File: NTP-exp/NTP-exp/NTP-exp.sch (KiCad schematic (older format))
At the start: 19 parts

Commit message: exp pcb
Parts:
- removed Q? (x2): 2N3904, Package_TO_SOT_SMD:SOT-23, symbol Transistor_BJT:2N3904
- removed R?: 10k, Resistor_SMD:R_0805_2012Metric_Pad1.15x1.40mm_HandSolder, symbol Device:R_US
- removed R? (x2): 1k, Resistor_SMD:R_0805_2012Metric_Pad1.15x1.40mm_HandSolder, symbol Device:R_US
- removed R?: 200, Resistor_SMD:R_0805_2012Metric_Pad1.15x1.40mm_HandSolder, symbol Device:R_US
- added D3, D4, D5, D6, D7: LED, LED_THT:LED_D3.0mm_FlatTop, symbol Device:LED
- added J10, J11, J12, J13, J14, J15, J16, J17, J18, J4, J5, J6, J7, J8, J9: PJ301M-12, eurorack:PJ301M-12, symbol Eurorack:PJ301M-12
- added R1, R10, R15, R18, R19, R20, R23, R24, R25, R28, R29, R30, R33, R34, R4, R5, R6, R9: 51, Resistor_SMD:R_0805_2012Metric_Pad1.15x1.40mm_HandSolder, symbol Device:R_US
- added R16, R21, R26, R31, R7: 10m, Resistor_SMD:R_0805_2012Metric_Pad1.15x1.40mm_HandSolder, symbol Device:R_US
- added R17, R22, R27, R3, R32, R8: 1k, Resistor_SMD:R_0805_2012Metric_Pad1.15x1.40mm_HandSolder, symbol Device:R_US
- added SW2: SW_Rotary3x4, Potentiometer_THT:Potentiometer_Alpha_RD901F-40-00D_Single_Vertical, symbol Switch:SW_Rotary3x4
- added U1, U2, U4, U5, U6, U7: TL074, Package_DIP:DIP-14_W7.62mm_Socket, symbol Amplifier_Operational:TL074
- D2: renamed from D?; footprint Display_7Segment:7SegmentLED_LTS6760_LTS6780 -> Display_7Segment:AFF_2x7SEG-DIGIT_10mm
- R2: renamed from R?; value 1k -> 10m
- SW1: renamed from SW?; footprint (none) -> Potentiometer_THT:Potentiometer_Alpha_RD901F-40-00D_Single_Vertical
- U3: renamed from U?; footprint Package_DIP:DIP-28_W7.62mm -> Package_DIP:DIP-28_W7.62mm_Socket
- gave numbers to parts that had none: 9
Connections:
- net labels added: STr4, STr5, STr6
- wire segments 25 -> 176
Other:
- moved on the sheet: D1, D2, H1, J1, J2, J3, R11, R12, R13, R14, R2, SW1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

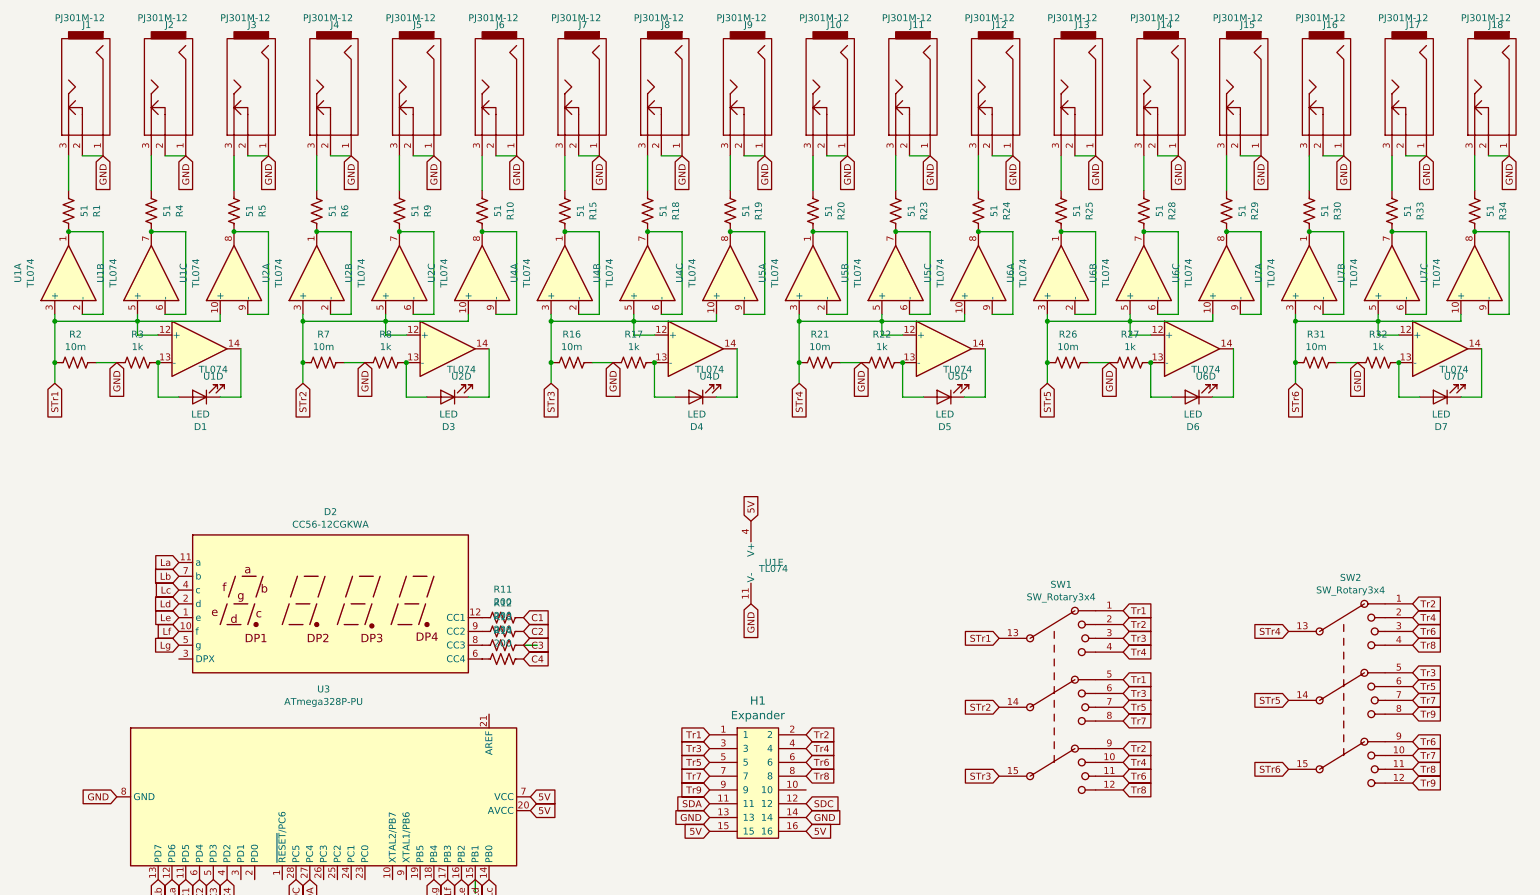
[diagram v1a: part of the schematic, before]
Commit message: designing
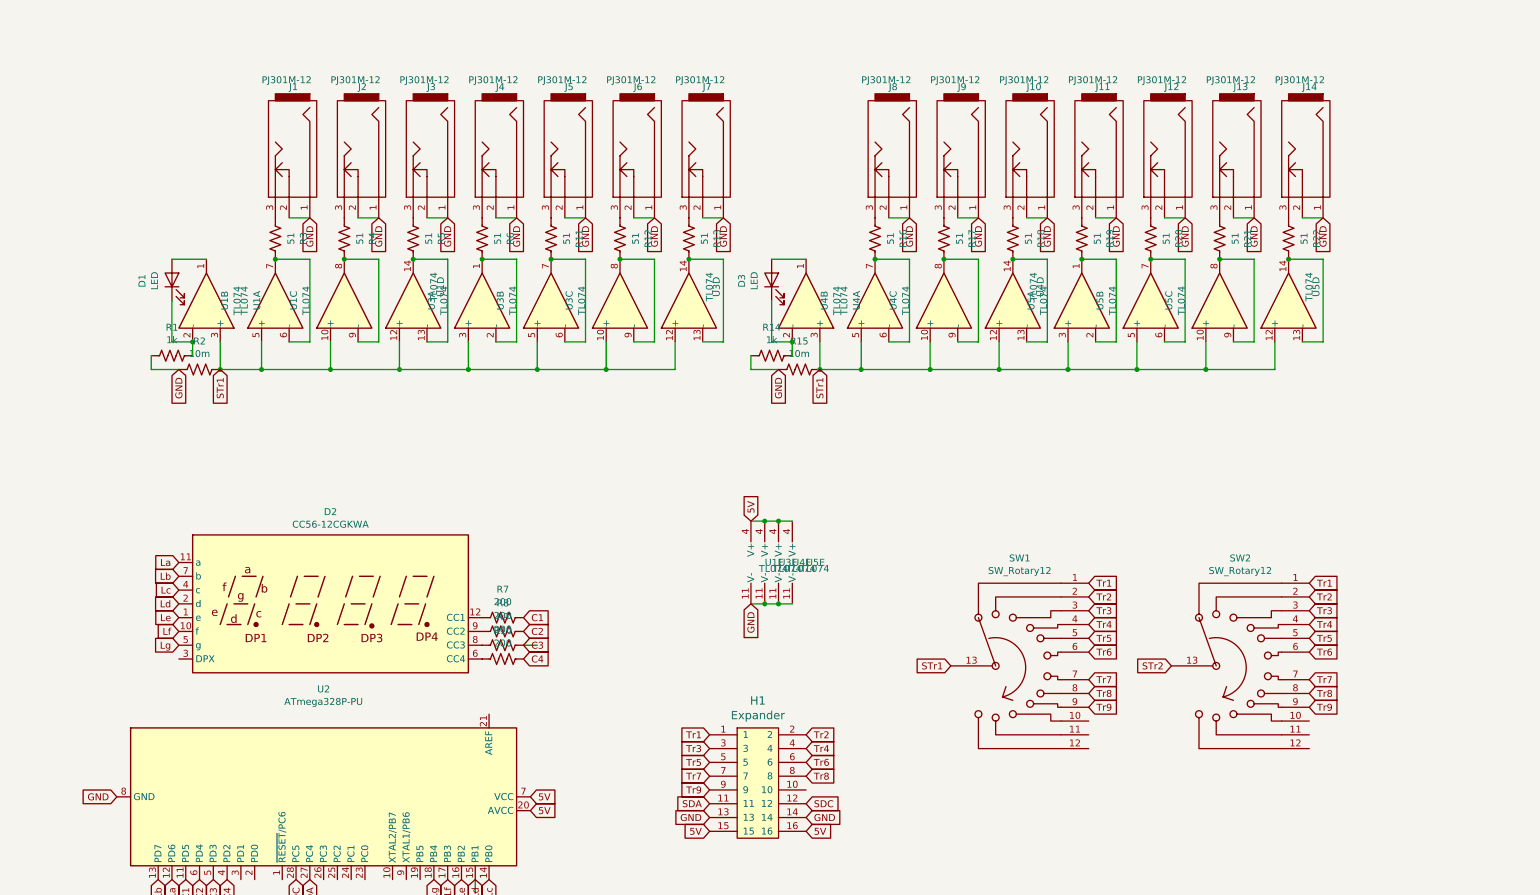
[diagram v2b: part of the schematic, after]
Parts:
- removed D4, D5, D6, D7: LED, LED_THT:LED_D3.0mm_FlatTop, symbol Device:LED
- removed J15, J16, J17, J18: PJ301M-12, eurorack:PJ301M-12, symbol Eurorack:PJ301M-12
- removed R10, R23, R24, R25, R28, R29, R30, R33, R34, R9: 51, Resistor_SMD:R_0805_2012Metric_Pad1.15x1.40mm_HandSolder, symbol Device:R_US
- removed R26, R31, R7: 10m, Resistor_SMD:R_0805_2012Metric_Pad1.15x1.40mm_HandSolder, symbol Device:R_US
- removed R27, R32, R8: 1k, Resistor_SMD:R_0805_2012Metric_Pad1.15x1.40mm_HandSolder, symbol Device:R_US
- removed SW1, SW2: SW_Rotary3x4, Potentiometer_THT:Potentiometer_Alpha_RD901F-40-00D_Single_Vertical, symbol Switch:SW_Rotary3x4
- removed U2, U6, U7: TL074, Package_DIP:DIP-14_W7.62mm_Socket, symbol Amplifier_Operational:TL074
- added R11, R12, R13: 51, Resistor_SMD:R_0805_2012Metric_Pad1.15x1.40mm_HandSolder, symbol Device:R_US
- added R14: 1k, Resistor_SMD:R_0805_2012Metric_Pad1.15x1.40mm_HandSolder, symbol Device:R_US
- added SW1, SW2: SW_Rotary12, symbol Switch:SW_Rotary12
- added U3: TL074, Package_DIP:DIP-14_W7.62mm_Socket, symbol Amplifier_Operational:TL074
- added unit 5 of U4
- added unit 5 of U5
- R1: value 51 -> 1k
- R15: value 51 -> 10m
- R16, R21: value 10m -> 51
- R17, R22, R3: value 1k -> 51
- renumbered R14 to R10, R11 to R7, R12 to R8, R13 to R9, U3 to U2
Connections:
- net 5V: now also U3.4 (V+), U4.4 (V+), U5.4 (V+)
- net GND: now also R1.2, R15.2, R2.2, R14.2, U3.11 (V-), U4.11 (V-), U5.11 (V-); no longer R16.1, R17.2, R2.1, R21.1, R22.2, R3.2
- net STr1: now also R15.1, R2.1, U4.10 (+), U4.12 (+), U4.3 (+), U4.5 (+), U5.10 (+), U5.12 (+), U5.3 (+), U5.5 (+), SW1.13, U3.10 (+), U3.12 (+), U3.3 (+), U3.5 (+); no longer R2.2
- net STr2: now also SW2.13
- net Tr1: now also SW1.1, SW2.1
- net Tr2: now also SW1.2, SW2.2
- net Tr3: now also SW1.3, SW2.3
- net Tr4: now also SW1.4, SW2.4
- net Tr5: now also SW1.5, SW2.5
- net Tr6: now also SW1.6, SW2.6
- net Tr7: now also SW1.7, SW2.7
- net Tr8: now also SW1.8, SW2.8
- net Tr9: now also SW1.9, SW2.9
- net at D1.1 (K): now also R1.1, U1.2 (-); no longer U1.14
- net at J1.3: now also R3.2; no longer R1.2
- net at U1.6 (-), U1.7: now also R3.1; no longer R4.1
- net at U1.8, U1.9 (-): now also R4.1; no longer R5.1
- net at D3.1 (K): now also U4.2 (-), R14.1
- net at D3.2 (A): now also U4.1
- net at J6.3: now also R12.2
- net at J5.3: now also R11.2
- net at R6.1: now also U3.1, U3.2 (-)
- net at U4.14: now also R18.1, U4.13 (-)
- net at R17.1: now also U4.8, U4.9 (-); no longer U4.13 (-)
- net at J9.3: now also R17.2; no longer R19.2
- net at J7.3: now also R13.2; no longer R15.2
- net at J8.3: now also R16.2; no longer R18.2
- net at U4.6 (-), U4.7: now also R16.1; no longer R18.1
- net at U5.14: now also R22.1, U5.13 (-)
- net at J12.3: now also R20.2
- net at J10.3: now also R18.2; no longer R20.2
- net at J11.3: now also R19.2
- net at U5.1, U5.2 (-): now also R19.1; no longer R20.1
- net at U5.6 (-), U5.7: now also R20.1
- net at U5.8, U5.9 (-): now also R21.1
- net at J13.3: now also R21.2
- net at J14.3: now also R22.2
- removed net STr3: R16.2, U4.10 (+), U4.12 (+), U4.3 (+), U4.5 (+)
- removed net STr4: R21.2, U5.10 (+), U5.12 (+), U5.3 (+), U5.5 (+)
- new net: D1.2 (A), U1.1
- new net: R5.1, U1.13 (-), U1.14
- new net: R11.1, U3.6 (-), U3.7
- new net: R12.1, U3.8, U3.9 (-)
- new net: R13.1, U3.13 (-), U3.14
